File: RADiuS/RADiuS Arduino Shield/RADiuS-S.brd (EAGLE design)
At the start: 68.6 x 53.3 mm, 15 parts, among them U1 ARDUINOR3-BPLACE

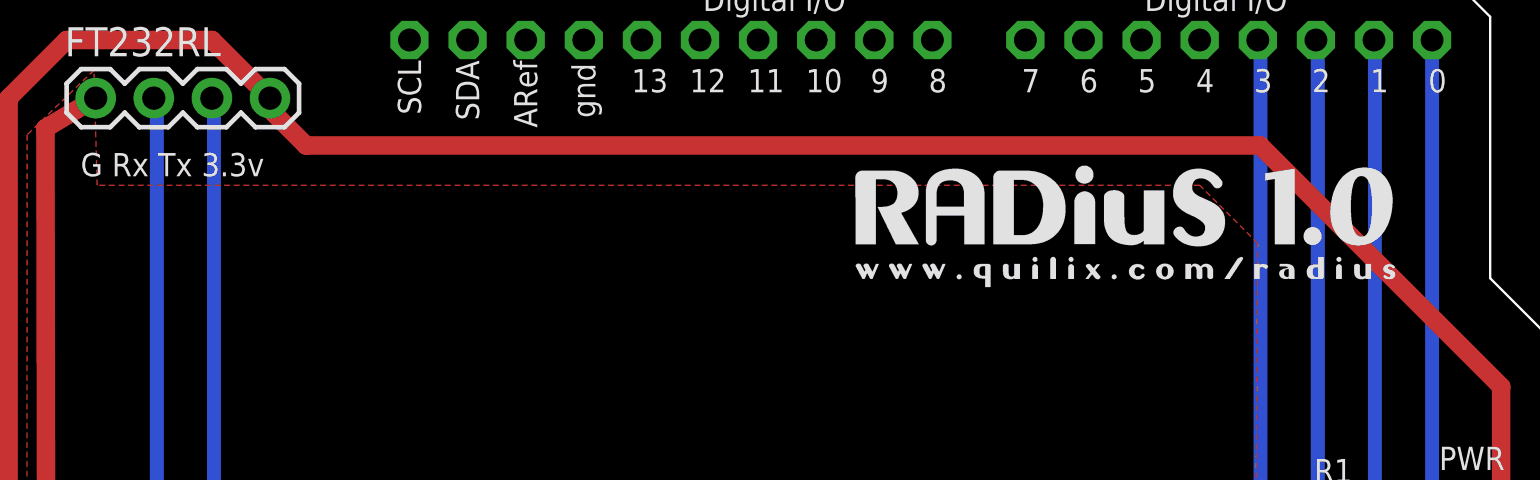
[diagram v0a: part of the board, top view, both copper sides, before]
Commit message: production update for RADiuS projects
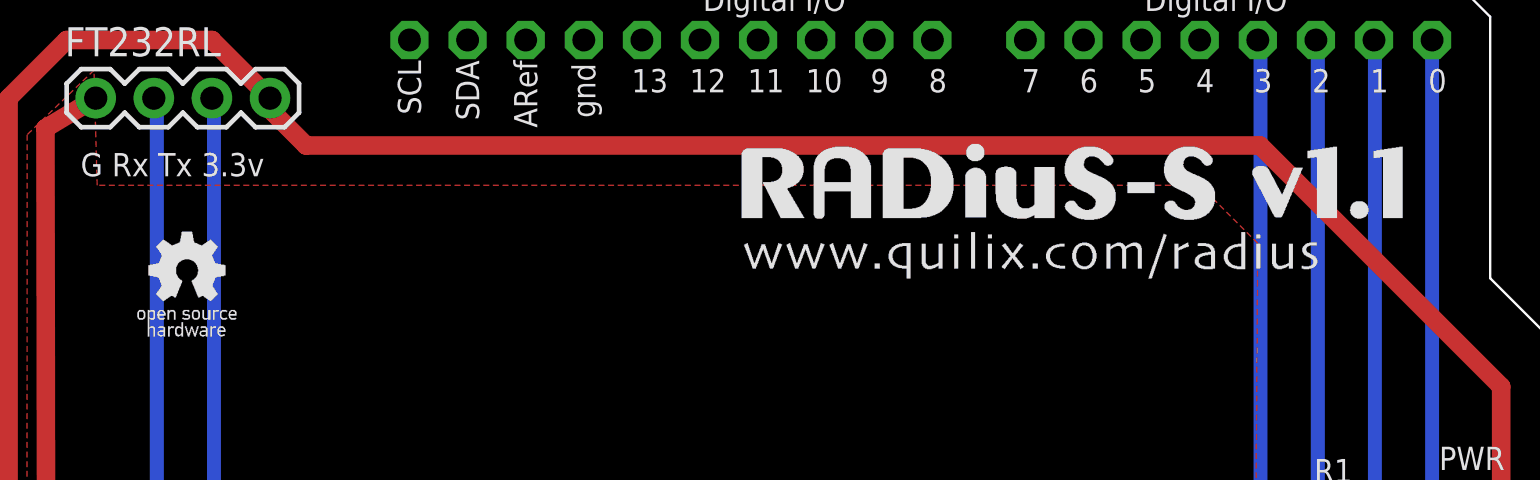
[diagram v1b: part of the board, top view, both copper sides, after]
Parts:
- R5, R6: value 330R -> 220R
